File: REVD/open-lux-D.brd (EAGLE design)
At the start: 54.4 x 53.2 mm, 51 parts, among them IC2 MCP73831, IC3 ATMEGA32U4-AU, IC4 MCP1700-33, J1 AYZ0202, Q4 BSS123, T1 FDN340P, T2 FDN340P, X2 USBSMD, X3 8MHz

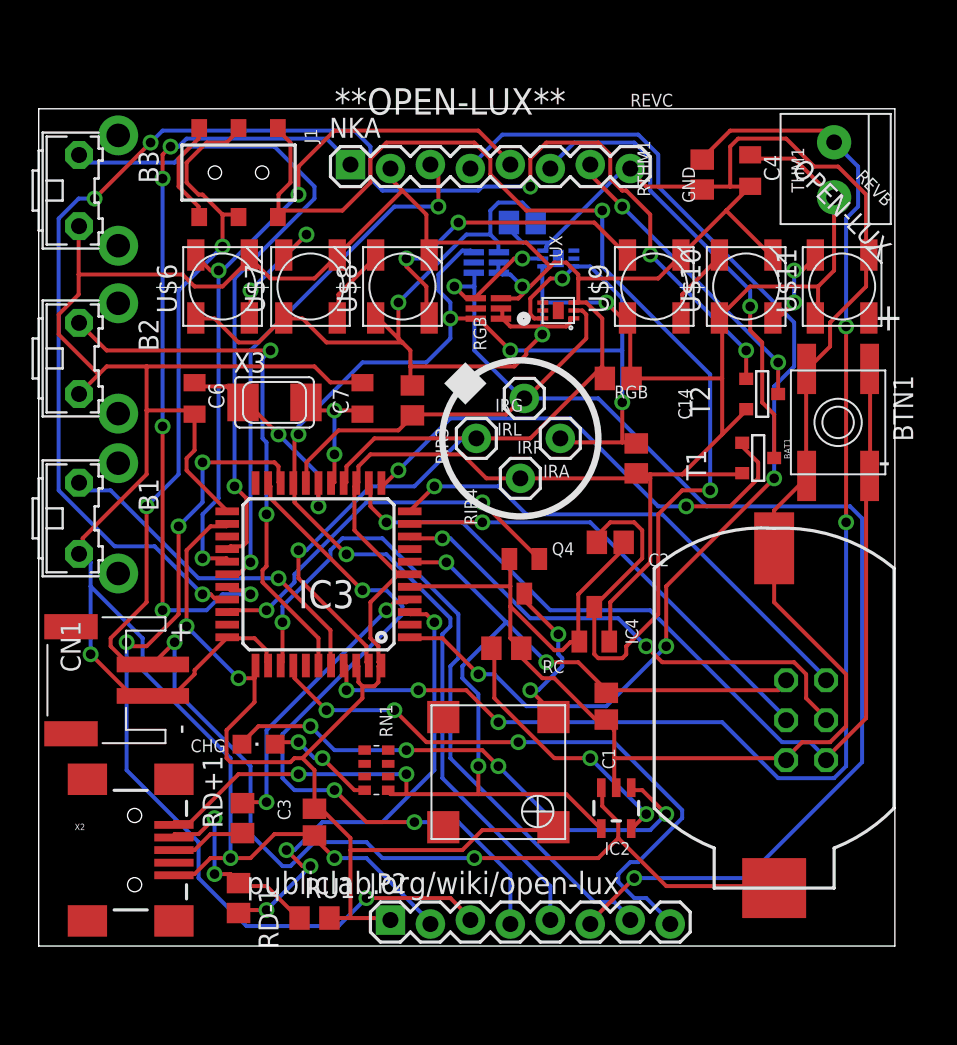
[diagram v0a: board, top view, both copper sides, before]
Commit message: update
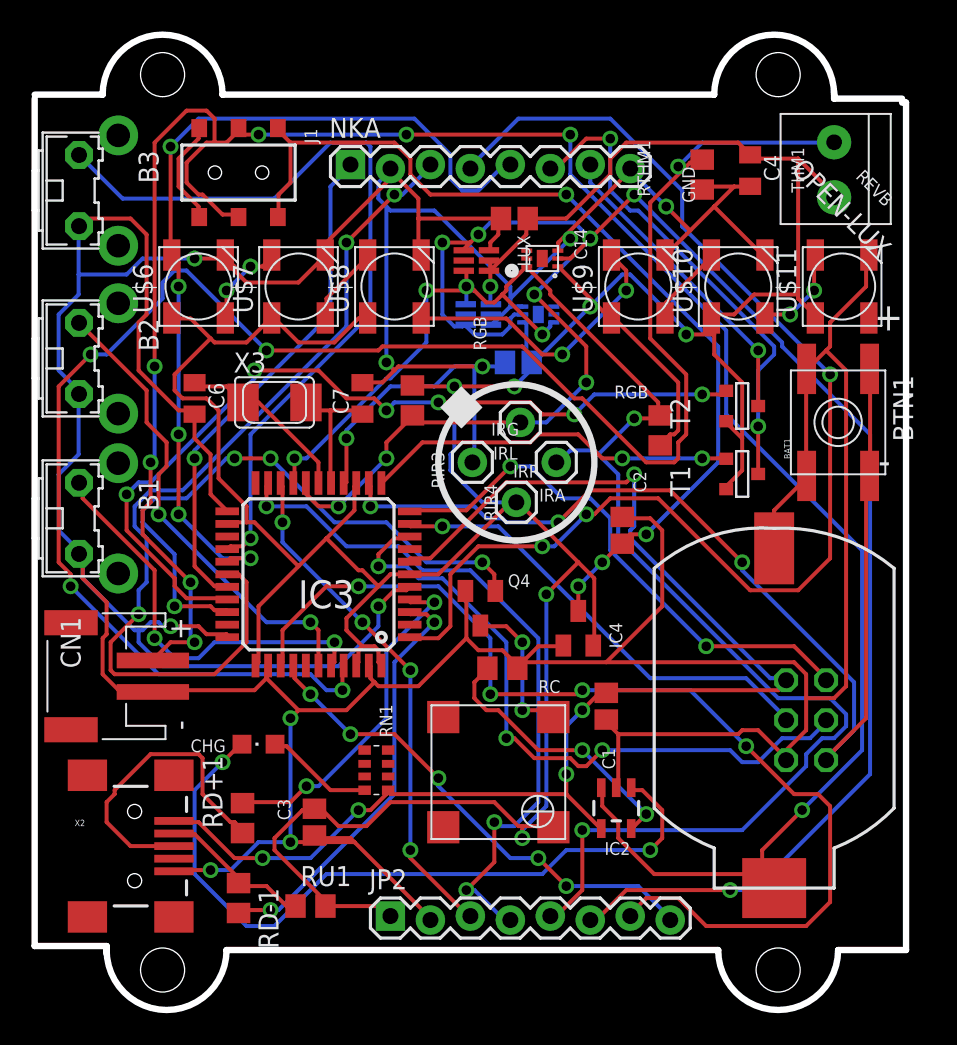
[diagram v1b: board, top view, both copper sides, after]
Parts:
- moved C14 12.1 mm to (30.2, 46.2)
- moved C5 8.89 mm to (30.5, 37.1)
- moved LUXRGB2 3.78 mm to (31.8, 40.1)
- moved LUXRGB1 3.45 mm to (32.0, 43.7)
- moved Q4 3.45 mm to (28.1, 21.5)
- moved LUXNIR1 3.34 mm to (27.9, 40.1)
- moved LUXNIR 3.14 mm to (27.8, 43.6)
- moved RIR4 2.34 mm to (39.5, 32.8)
- moved IRL 1.55 mm to (30.6, 33.3)
- moved IRA 1.55 mm to (32.9, 30.7)
- moved IRG 1.55 mm to (27.6, 30.7)
- moved IRP 1.55 mm to (30.4, 28.2)
- moved U$6 1.52 mm to (10.2, 41.9)
- moved T2 1.48 mm to (44.7, 34.3)
- moved T1 1.44 mm to (44.7, 30.0)
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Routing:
- net VBAT: track 100.3 -> 148.1 mm, vias 4 -> 8
- net D10: track 91.6 -> 54.8 mm
- net GND: track 361.2 -> 390.9 mm, vias 5 -> 11
- net A5: track 86.3 -> 115.9 mm
- net SCL: track 104.2 -> 129.4 mm, vias 3 -> 9
- net RXD: track 57.4 -> 32.7 mm
- net D8: track 33.9 -> 57.5 mm, vias 2 -> 3
- net VCC: track 227.7 -> 250.6 mm, vias 5 -> 7
- net A0: track 44.2 -> 67.0 mm, vias 1 -> 4
- net VDD: track 81.9 -> 60.6 mm, vias 2 -> 4
- net D9: track 49.8 -> 32.2 mm, vias 5 -> 1
- net D+: track 4.84 -> 19.8 mm
- net D5: track 24.5 -> 38.3 mm, vias 2 -> 4
- net N$5: track 33.5 -> 47.3 mm, vias 4 -> 2
- net VBUS: track 72.3 -> 85.3 mm
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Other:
- board size 54.4 x 53.2 mm -> 55.4 x 62 mm
